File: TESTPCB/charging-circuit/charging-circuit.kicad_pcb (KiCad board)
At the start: 2 copper layers, 82.6 x 94.6 mm, 271 parts, among them J1 2.54-1*6PHeader-RA, J10 Conn_01x02, J11 Conn_01x04, J2 USB_C_Receptacle_PowerOnly_6P, P1 Header-Male-2.54_2x2, P10 1.27mm/1*3p, P11 1.27mm/1*3p, P2 Header-Male-2.54_2x2, P3 1.27mm/1*3p, P4 1.27mm/1*3p, P5 1.27mm/1*3p, P6 1.27mm/1*3p, P7 1.27mm/1*3p, P8 1.27mm/1*3p, P9 1.27mm/1*3p, Q1 2N7002, Q10 AO3400A, Q11 AO3401A, Q2 CJQ4435, Q3 currentmirror, Q4 BSS84, Q5 AO4892, Q6 AO3401A, Q7 AO3401A, Q8 CJQ4435, Q9 AO3400A, SW1 TS-1088R-02026, U1 MAX17048G+T10, U10 BQ25606RGER, U11 Battery Input, U12 BQ24170RGYR, U13 TPS54302DDCR_C311983, U14 NTC10K/0805/F, U15 BQ76920PW, U16 NTC10K/0805/F, U17 HUSB238_002DD, U19 TPS54302DDCR_C311983, U2 MT3608, U20 TPS54302DDCR_C311983, U21 MCP73871, U22 SRP4020TA-1R0M, U3 MT3608, U4 TPL5110DDCT, U5 BQ25606RGER, U6 MT3608, U7 Z-21320110021001, U8 MAX3232CDBR, U9 ADS1115IDGSR

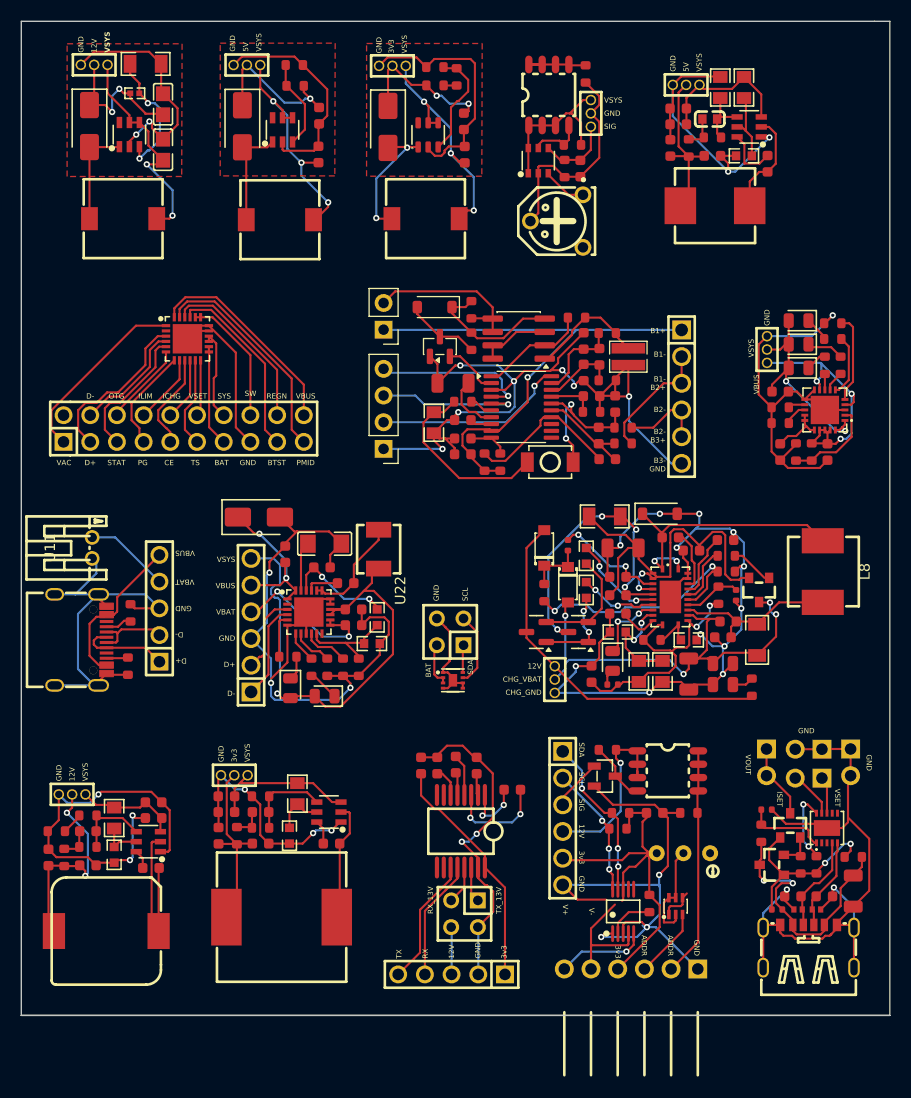
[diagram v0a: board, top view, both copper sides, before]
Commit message: fixed drc
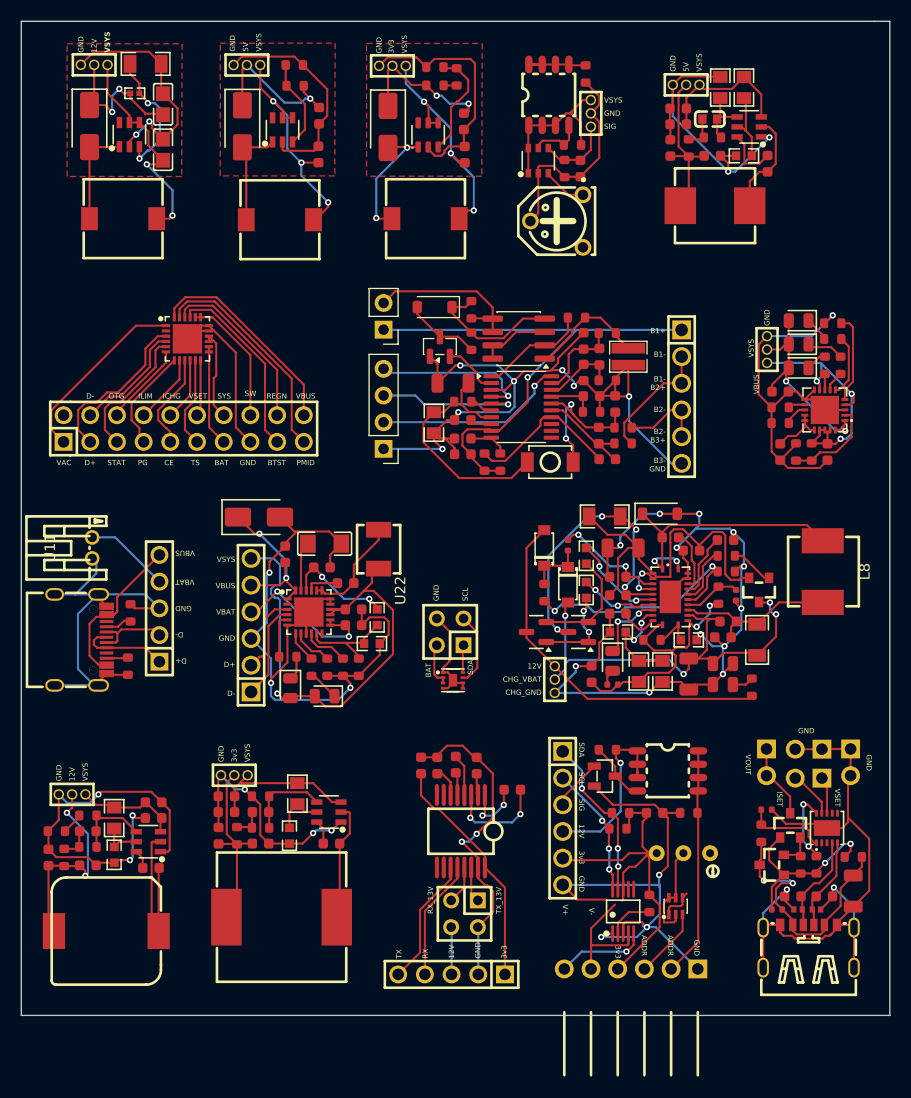
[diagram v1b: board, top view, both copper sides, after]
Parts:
- removed the ? at (72.7, 31.4)
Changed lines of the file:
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@@
 	(footprint ""
 		(layer "F.Cu")
-		(at 72.675 31.45 90)
-		(property "Reference" ""
-			(at 0 0 90)
-			(layer "F.SilkS")
-			(effects
-				(font
-					(size 1.27 1.27)
-					(thickness 0.15)
-				)
-			)
-		)
-		(property "Value" ""
-			(at 0 0 90)
-			(layer "F.Fab")
-			(effects
-				(font
-					(size 1.27 1.27)
-					(thickness 0.15)
-				)
-			)
-		)
-		(property "Datasheet" ""
-			(at 0 0 90)
-			(layer "F.Fab")
-			(hide yes)
-			(effects
-				(font
-					(size 1.27 1.27)
-					(thickness 0.15)
-				)
-			)
-		)
-		(property "Description" ""
-			(at 0 0 90)
-			(layer "F.Fab")
-			(hide yes)
-			(effects
-				(font
-					(size 1.27 1.27)
-					(thickness 0.15)
-				)
-			)
-		)
-		(pad "" np_thru_hole circle
-			(at 0 0 180)
-			(size 0.5 0.5)
-			(drill oval 0.5 23)
-			(layers "*.Cu" "*.Mask")
-		)
-		(embedded_fonts no)
-	)
-	(footprint ""
-		(layer "F.Cu")
 		(at 58.525 31.5 90)
 		(property "Reference" ""
@@
 		(stroke
 			(width 0.05)
-			(type default)
-		)
-		(layer "Edge.Cuts")
-	)
-	(gr_line
-		(start 109.79 114.18)
-		(end 27.15 114.18)
-		(stroke
-			(width 0.05)
